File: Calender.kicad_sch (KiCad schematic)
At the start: 35 parts, among them J1 Screen, J2 USB_C_Receptacle_USB2.0_16P, J3 Power, SW1 RotaryEncoder_Switch, SW2 SW_Push, SW3 SW_Push, SW4 SW_Push, U1 ATSAMD21G18A-A, U3 MCP73871, U4 AMS1117-3.3, U5 ESP-WROOM-02

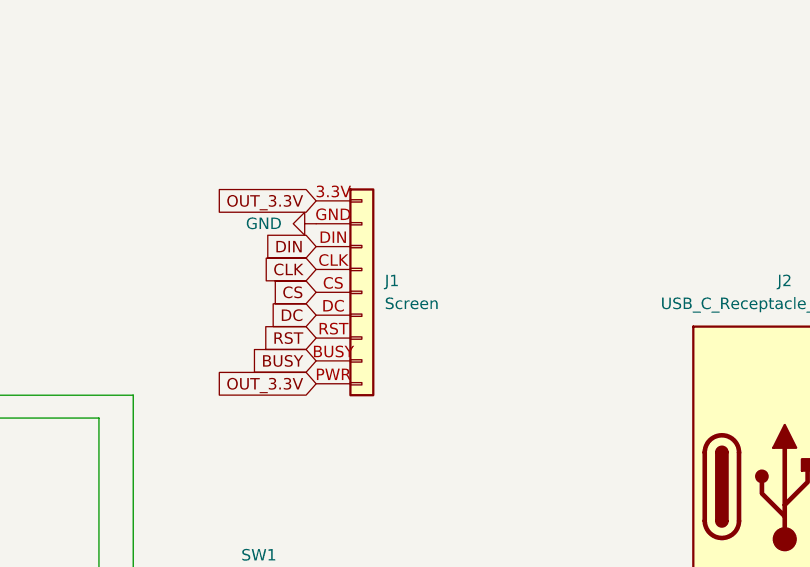
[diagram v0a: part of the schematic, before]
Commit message: all routing and stuff... definitely didn't forget to push
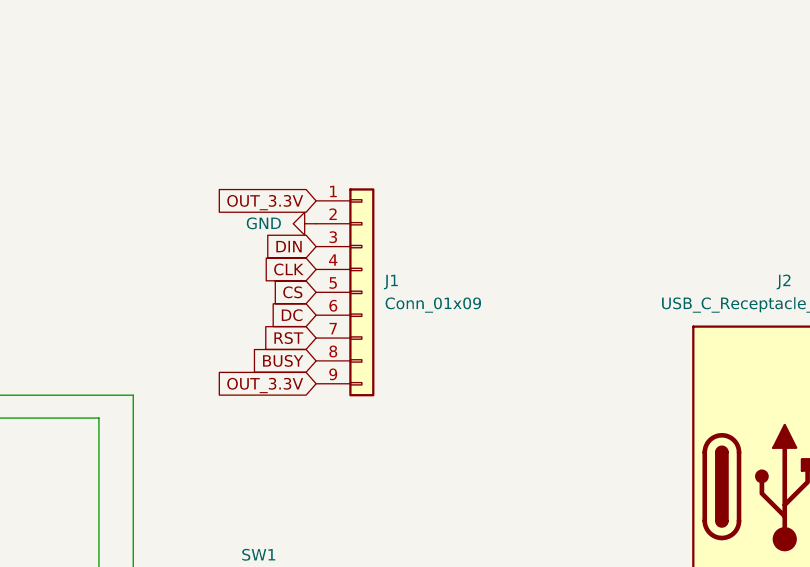
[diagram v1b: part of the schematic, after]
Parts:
- C10, C11, C5, C6, C7, C8, C9: footprint (none) -> Capacitor_SMD:C_0603_1608Metric
- J1: value Screen -> Conn_01x09; footprint Connector_PinHeader_2.54mm:PinHeader_1x09_P2.54mm_Vertical_SMD_Pin1Right -> Connector_PinHeader_1.00mm:PinHeader_1x09_P1.00mm_Vertical
- J3: footprint Connector_Phoenix_SPT:PhoenixContact_SPT_1.5_2-H-3.5_1x02_P3.5mm_Horizontal -> TerminalBlock:TerminalBlock_bornier-2_P5.08mm
- SW2, SW3, SW4: footprint (none) -> Button_Switch_THT:SW_PUSH_6mm
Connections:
- net BUSY: now also J1.8 (Pin_8); no longer J1.BUSY (IO25)
- net CLK: now also J1.4 (Pin_4); no longer J1.CLK (IO13)
- net CS: now also J1.5 (Pin_5); no longer J1.CS (IO15)
- net DC: now also J1.6 (Pin_6); no longer J1.DC (1O27)
- net DIN: now also J1.3 (Pin_3); no longer J1.DIN (IO14)
- net GND: now also J1.2 (Pin_2); no longer J1.GND (Pin_2)
- net OUT_3.3V: now also J1.1 (Pin_1), J1.9 (Pin_9); no longer J1.3.3V (VCC), J1.PWR (IO33)
- net RST: now also J1.7 (Pin_7); no longer J1.RST (IO26)
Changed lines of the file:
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@@
 			)
 		)
-		(property "Footprint" ""
+		(property "Footprint" "Capacitor_SMD:C_0603_1608Metric"
 			(at 53.34 26.3652 0)
 			(effects
@@
 			)
 		)
-		(property "Footprint" ""
+		(property "Footprint" "Capacitor_SMD:C_0603_1608Metric"
 			(at 71.12 18.0848 0)
 			(effects
@@
 			)
 		)
-		(property "Footprint" ""
+		(property "Footprint" "Capacitor_SMD:C_0603_1608Metric"
 			(at 64.4652 134.62 0)
 			(effects
@@
 			)
 		)
-		(property "Footprint" ""
+		(property "Footprint" "Capacitor_SMD:C_0603_1608Metric"
 			(at 71.12 23.1648 0)
 			(effects
@@
 			)
 		)
-		(property "Value" "Screen"
+		(property "Value" "Conn_01x09"
 			(at 133.35 48.2599 0)
 			(effects
@@
 			)
 		)
-		(property "Footprint" "Connector_PinHeader_2.54mm:PinHeader_1x09_P2.54mm_Vertical_SMD_Pin1Right"
+		(property "Footprint" "Connector_PinHeader_1.00mm:PinHeader_1x09_P1.00mm_Vertical"
 			(at 130.81 46.99 0)
 			(effects
@@
 			)
 		)
-		(pin "DIN"
+		(pin "7"
 		)
-		(pin "BUSY"
+		(pin "5"
 		)
-		(pin "3.3V"
+		(pin "2"
 		)
-		(pin "RST"
+		(pin "8"
 		)
-		(pin "CLK"
+		(pin "6"
 		)
-		(pin "DC"
+		(pin "9"
 		)
-		(pin "CS"
+		(pin "1"
 		)
-		(pin "PWR"
+		(pin "4"
 		)
-		(pin "GND"
+		(pin "3"
 		)
 		(instances
@@
 			)
 		)
-		(property "Footprint" ""
+		(property "Footprint" "Button_Switch_THT:SW_PUSH_6mm"
 			(at 266.7 135.89 0)
 			(effects
@@
 			)
 		)
-		(property "Footprint" ""
+		(property "Footprint" "Button_Switch_THT:SW_PUSH_6mm"
 			(at 92.71 114.3 0)
 			(effects
@@
 			)
 		)
-		(property "Footprint" "Connector_Phoenix_SPT:PhoenixContact_SPT_1.5_2-H-3.5_1x02_P3.5mm_Horizontal"
+		(property "Footprint" "TerminalBlock:TerminalBlock_bornier-2_P5.08mm"
 			(at 130.81 102.87 0)
 			(effects
@@
 			)
 		)
-		(property "Footprint" ""
+		(property "Footprint" "Capacitor_SMD:C_0603_1608Metric"
 			(at 45.72 31.4452 0)
 			(effects
@@
 			)
 		)
-		(property "Footprint" ""
+		(property "Footprint" "Capacitor_SMD:C_0603_1608Metric"
 			(at 55.88 17.4752 0)
 			(effects
@@
 			)
 		)
-		(property "Footprint" ""
+		(property "Footprint" "Button_Switch_THT:SW_PUSH_6mm"
 			(at 110.49 114.3 0)
 			(effects
@@
 			)
 		)
-		(property "Footprint" ""
+		(property "Footprint" "Capacitor_SMD:C_0603_1608Metric"
 			(at 55.88 22.5552 0)
 			(effects
